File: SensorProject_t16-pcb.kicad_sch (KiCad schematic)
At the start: 51 parts, among them J1 Conn_01x02_Pin, J10 Conn_01x02_Pin, J11 Conn_01x02_Pin, J12 Conn_01x02_Pin, J13 Conn_01x02_Pin, J14 Conn_01x02_Pin, J15 Conn_01x02_Pin, J16 Conn_01x02_Pin, J17 Conn_01x04_Socket, J2 Conn_01x02_Pin, J3 Conn_01x02_Pin, J4 Conn_01x02_Pin, J5 Conn_01x02_Pin, J6 Conn_01x02_Pin, J7 Conn_01x02_Pin, J8 Conn_01x02_Pin, J9 Conn_01x02_Pin, U1 ADS1115IDGS, U2 ADS1115IDGS, U3 ADS1115IDGS, U4 ADS1115IDGS

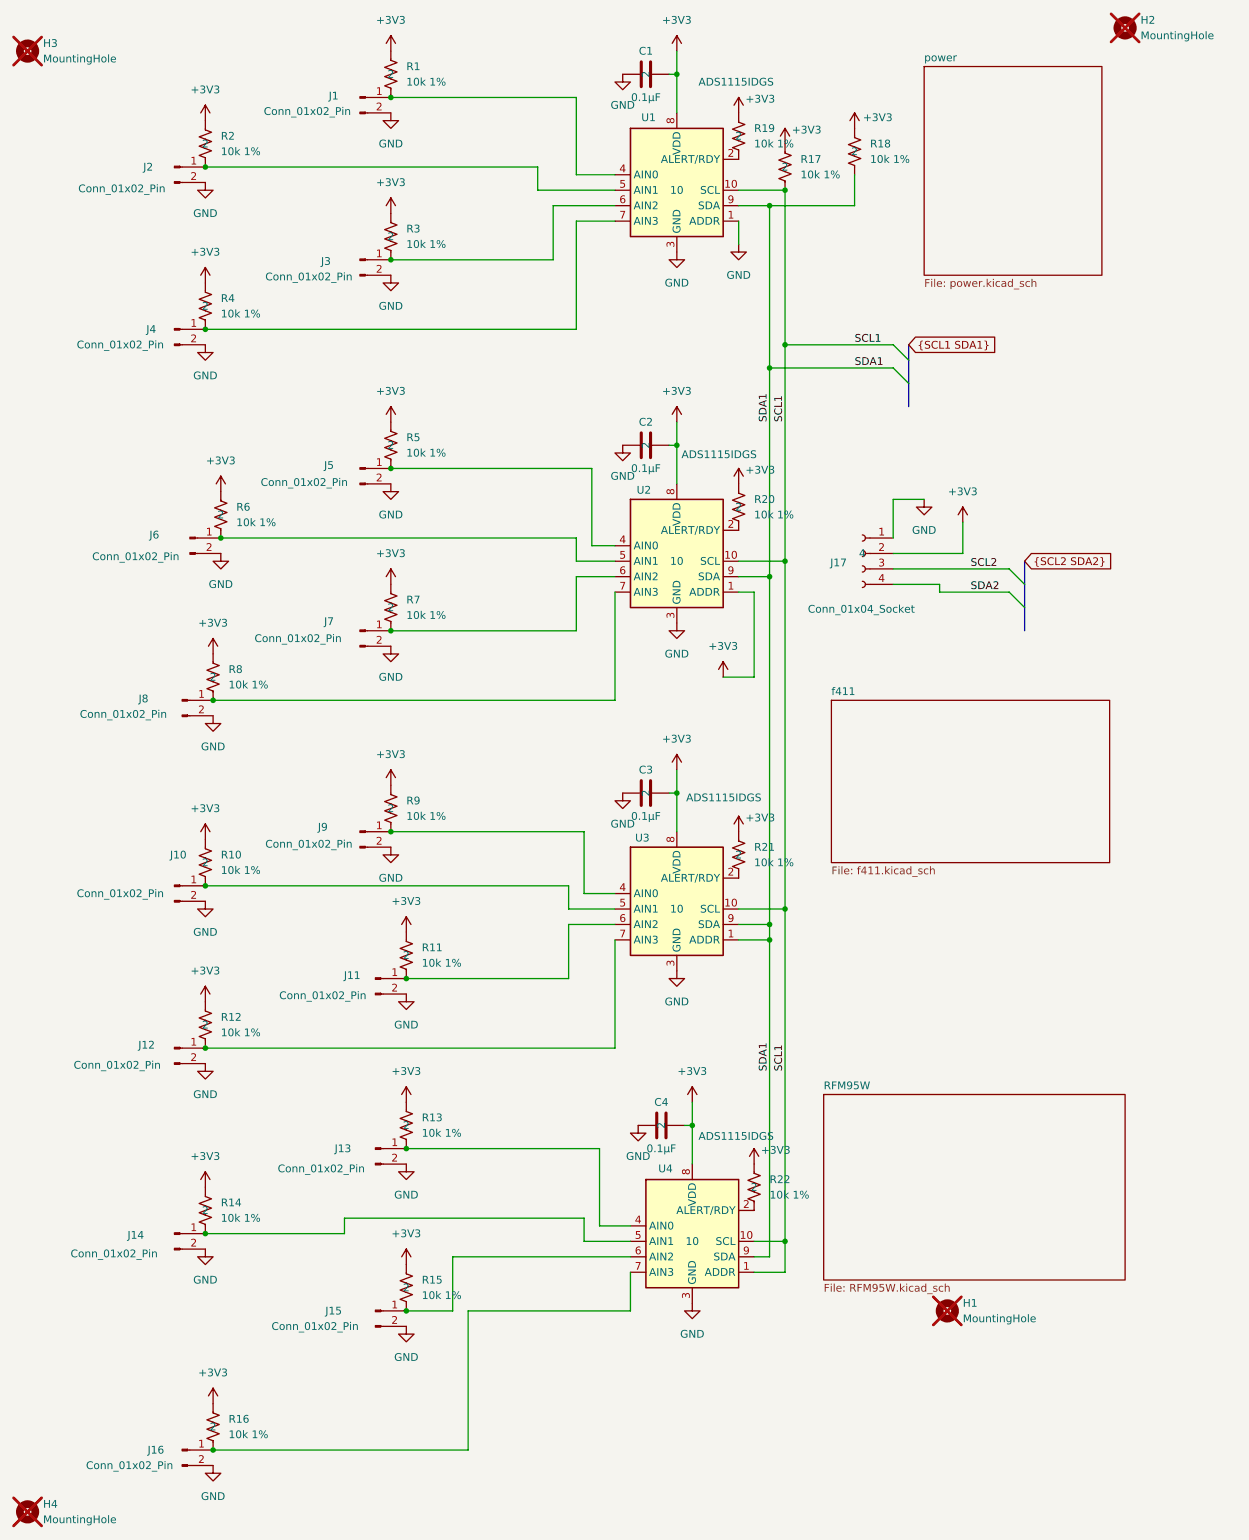
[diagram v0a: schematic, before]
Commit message: cleanup, ready to submit.
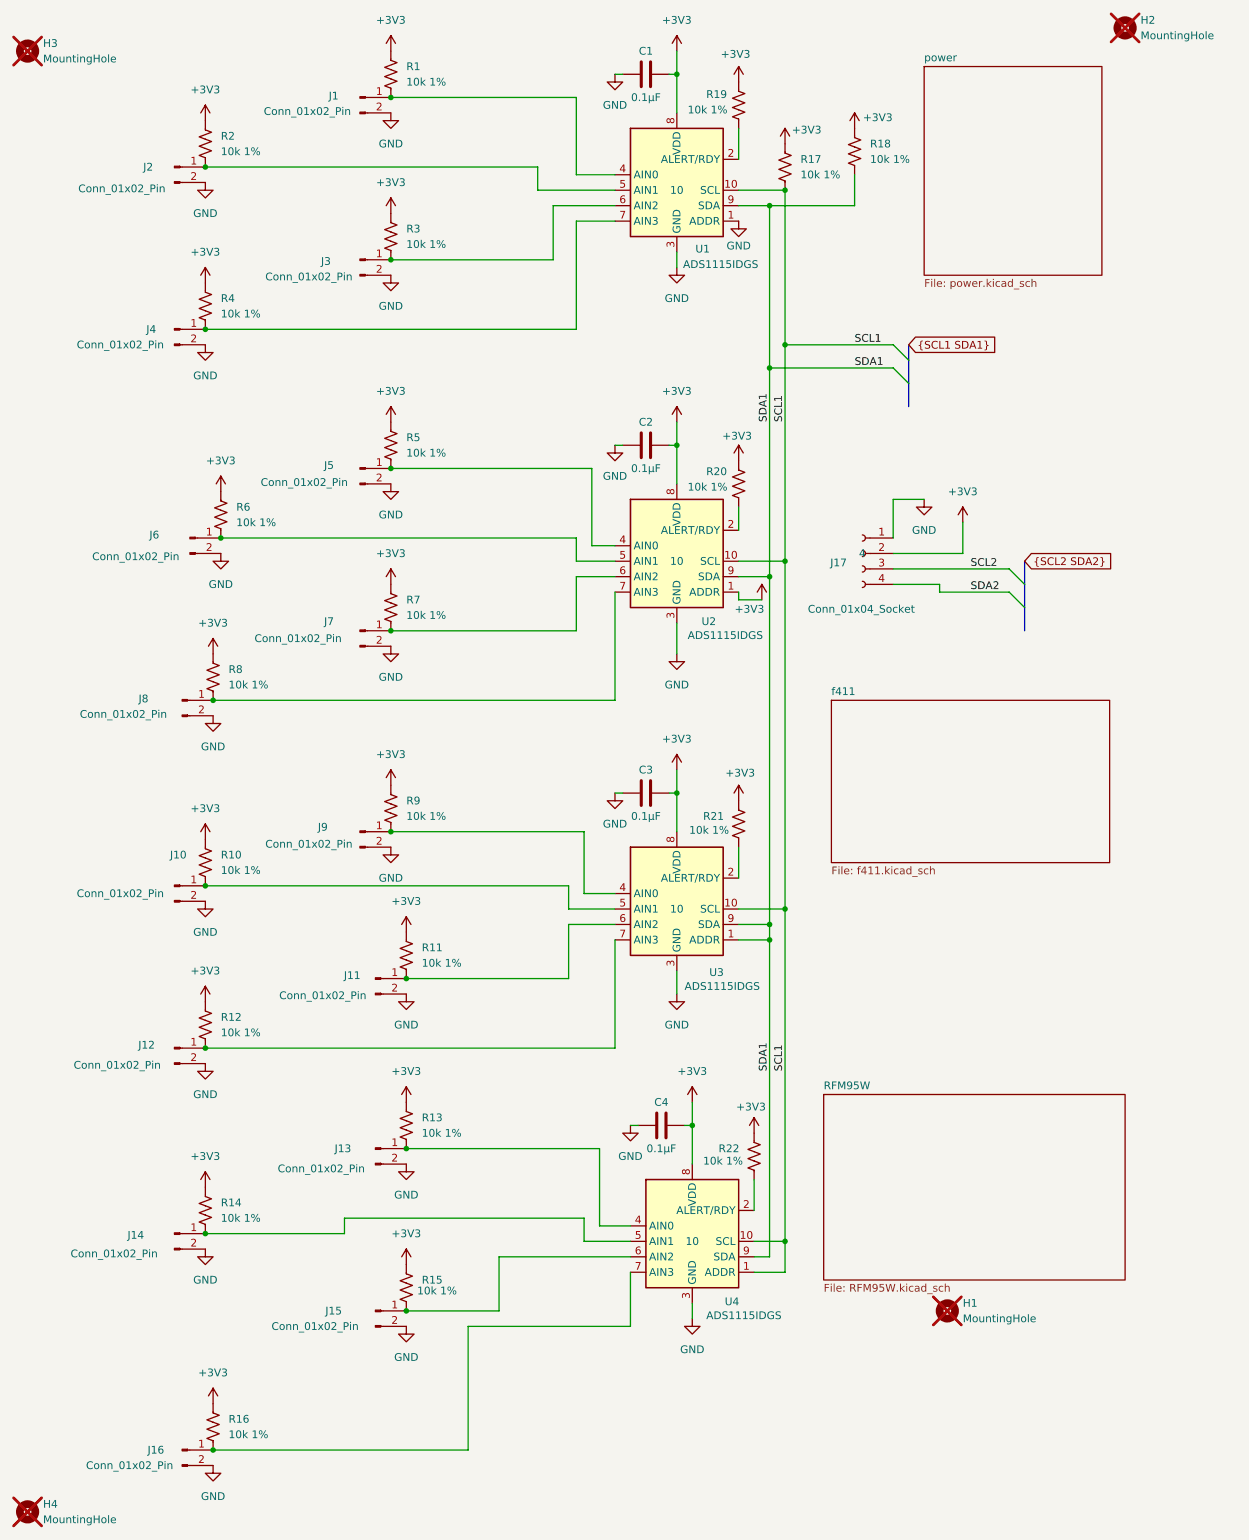
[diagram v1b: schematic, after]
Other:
- moved on the sheet: R19, R20, R21, R22
